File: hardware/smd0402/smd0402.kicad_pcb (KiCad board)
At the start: 2 copper layers, 150 x 98.6 mm, 118 parts, among them J1 Conn_01x03, J2 SAO v1.69bis addon, U1 WCH CH32V003F4U6

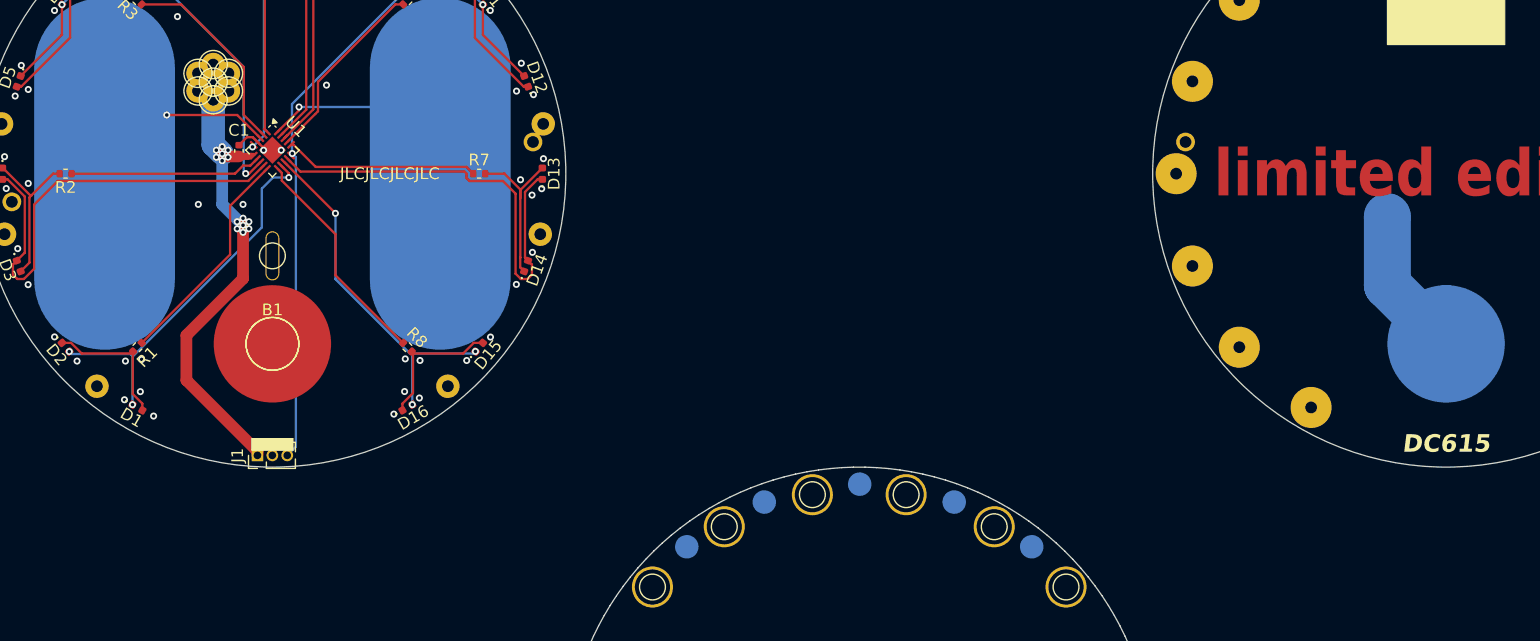
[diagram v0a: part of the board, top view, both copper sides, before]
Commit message: clean up DRC
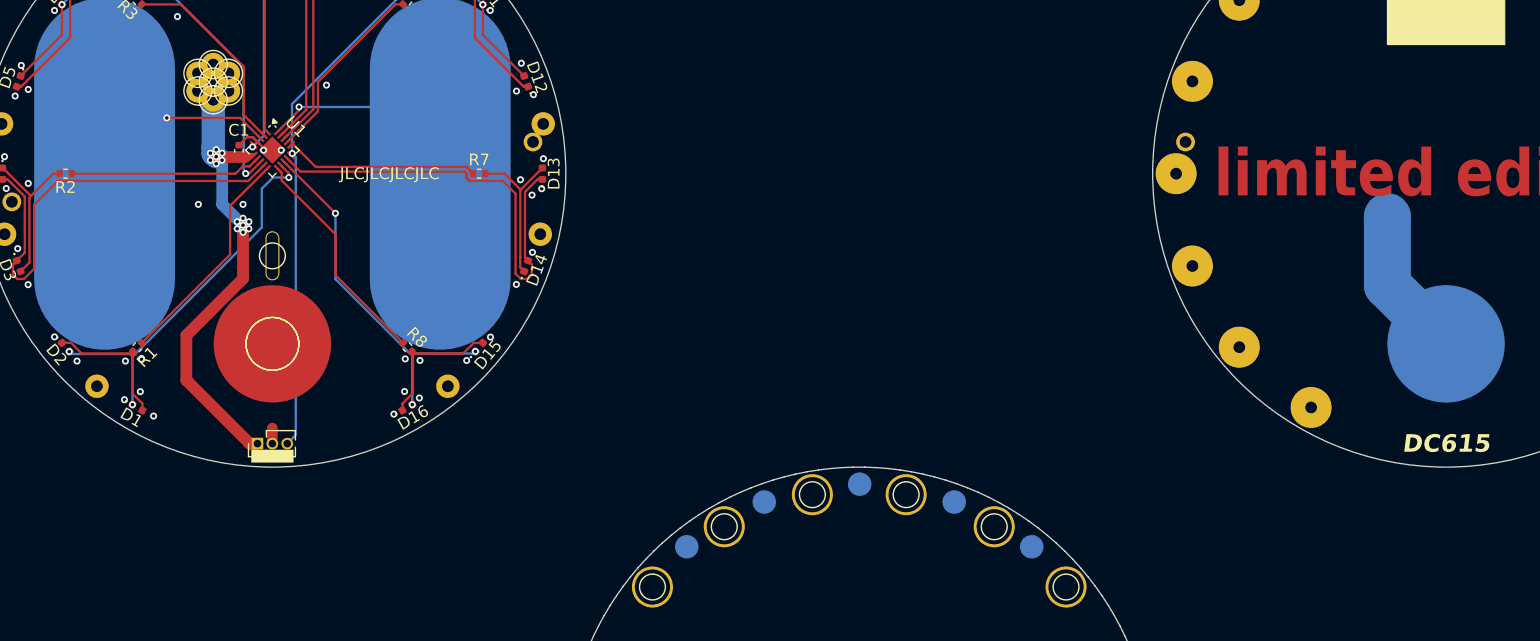
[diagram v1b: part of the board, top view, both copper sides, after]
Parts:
- moved B2 3.00 mm to (150.0, 114.5)
- moved J1 1.00 mm to (48.7, 123.0)
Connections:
- stitch2 pad 1: (no net) -> GND (x10)
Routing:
- net GND: track 25.4 -> 26.7 mm
- net GP6: track 58.6 -> 57.6 mm
- net Net-(D13-A): track 14.0 -> 13.3 mm
- net +3V0: track 83.5 -> 84.1 mm
